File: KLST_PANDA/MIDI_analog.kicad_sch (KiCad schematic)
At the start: 10 parts, among them J1 MIDI IN, J2 MIDI OUT, U1 H11L1SR2M, U2 74AHC1G125

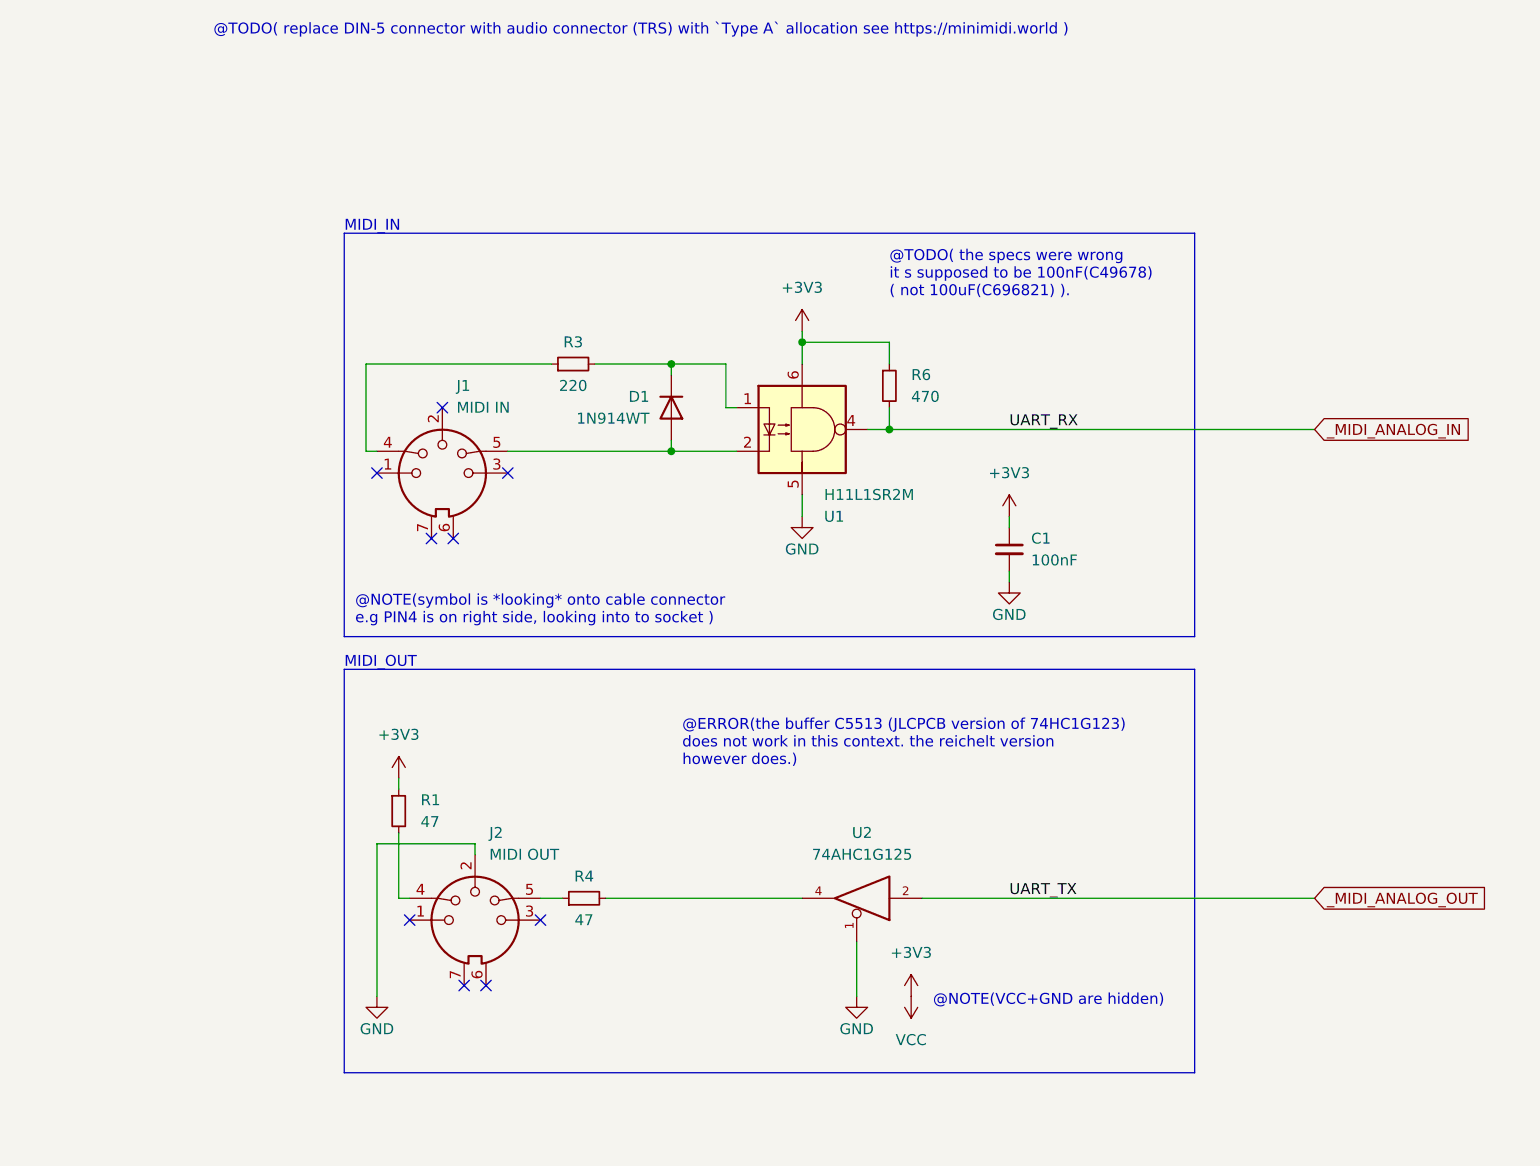
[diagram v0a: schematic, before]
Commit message: cleaned up main sheet
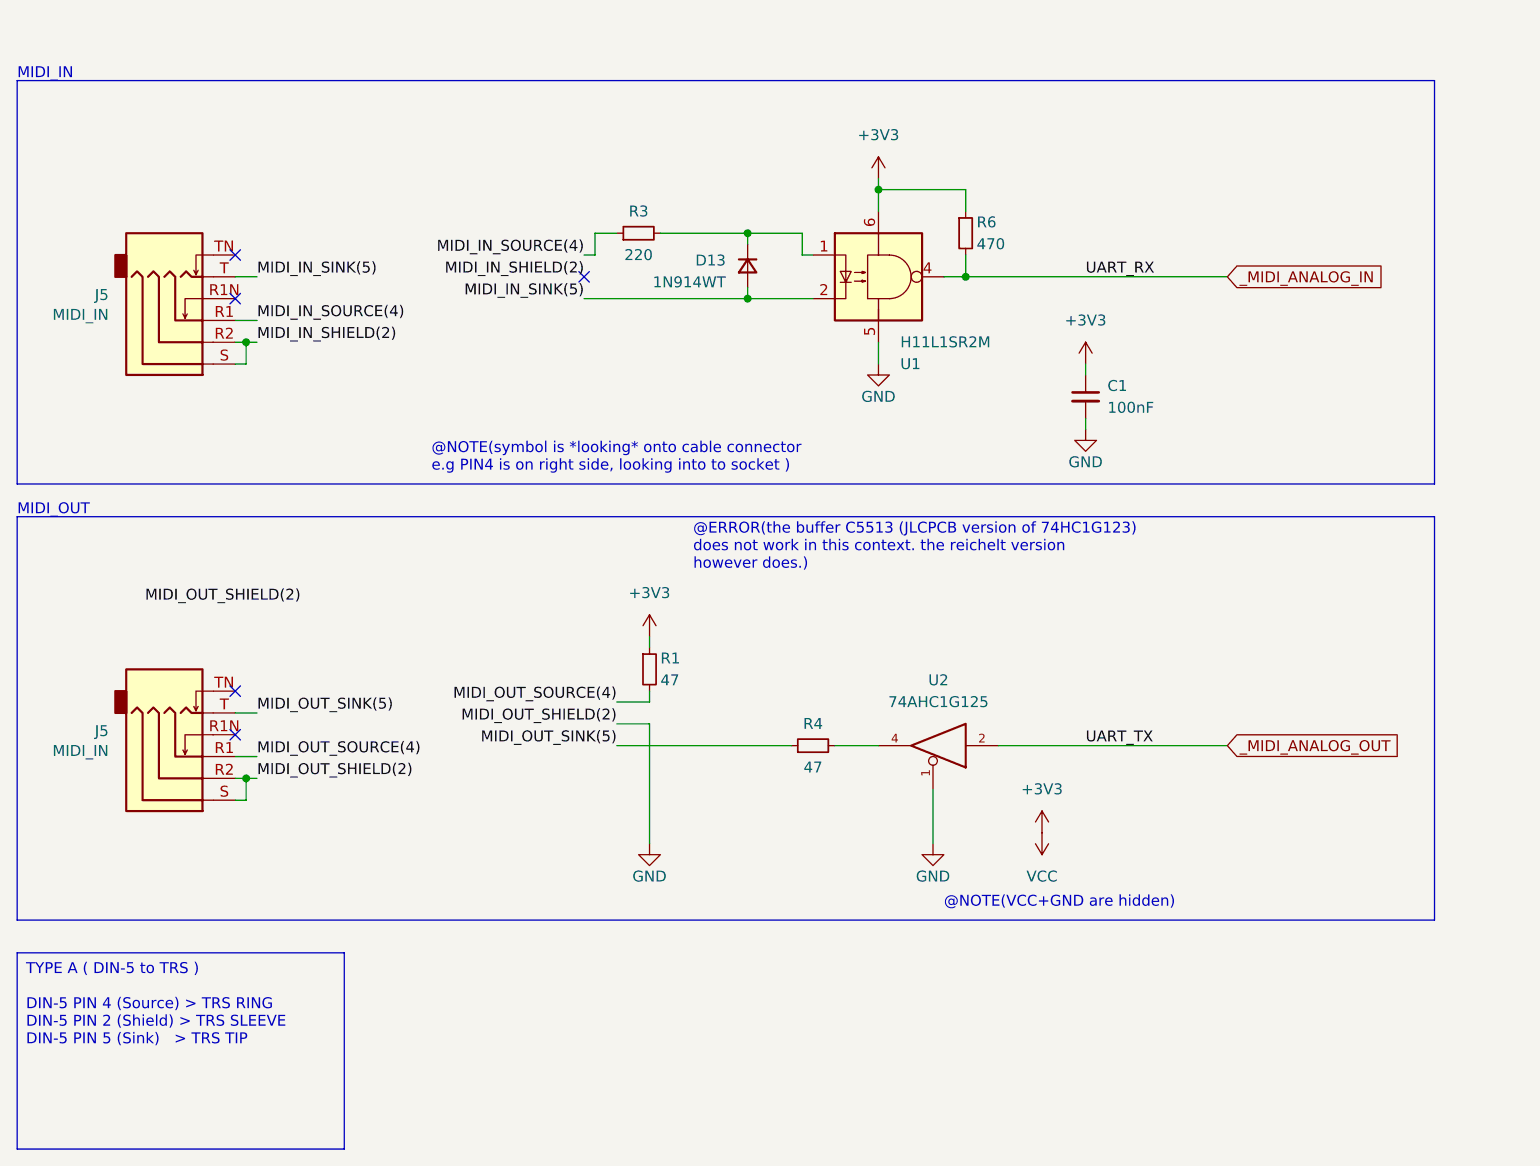
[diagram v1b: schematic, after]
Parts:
- removed D1: 1N914WT, Diode_SMD:D_SOD-523, symbol Diode:1N914WT
- removed J1: MIDI IN, DIN-5:DIN5-RA-PTH, symbol Connector:DIN-5_180degree_with_Eaerth
- removed J2: MIDI OUT, DIN-5:DIN5-RA-PTH, symbol Connector:DIN-5_180degree_with_Eaerth
- added D13: 1N914WT, Diode_SMD:D_SOD-523, symbol Device:D_Small
- added J5 (x2): MIDI_IN, KLST_SHEEP:Korean_Hroparts_Elec_PJ-316A-6A, symbol Connector:AudioJack4_SwitchTR1
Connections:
- net GND: now also J5.R2, J5.S
- net MIDI_OUT_SINK(5): now reaches R4.1
- net MIDI_OUT_SINK(5): now also J5.T
- net MIDI_OUT_SOURCE(4): now reaches R1.2
- net MIDI_OUT_SOURCE(4): now also J5.R1
- net MIDI_IN_SOURCE(4): now reaches R3.1
- net MIDI_IN_SOURCE(4): now also J5.R1
- net at R3.2, U1.1: now also D13.1 (K)
- net MIDI_IN_SINK(5): now reaches U1.2
- net MIDI_IN_SINK(5): now also D13.2 (A), J5.T
- new net MIDI_IN_SHIELD(2): J5.R2, J5.S
- no-connect marks 9 -> 5
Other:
- note removed: "@TODO( replace DIN-5 connector with audio connector (TRS) with `Type A` allocation see https://minimidi.world )"
- note removed: "@TODO( the specs were wrong it s supposed to be 100nF(C49678) ( not 100uF(C696821) )."
- moved on the sheet: C1, R1, R3, R4, R6, U1, U2
